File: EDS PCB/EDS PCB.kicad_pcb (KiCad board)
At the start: 2 copper layers, 100 x 100 mm, 1 part

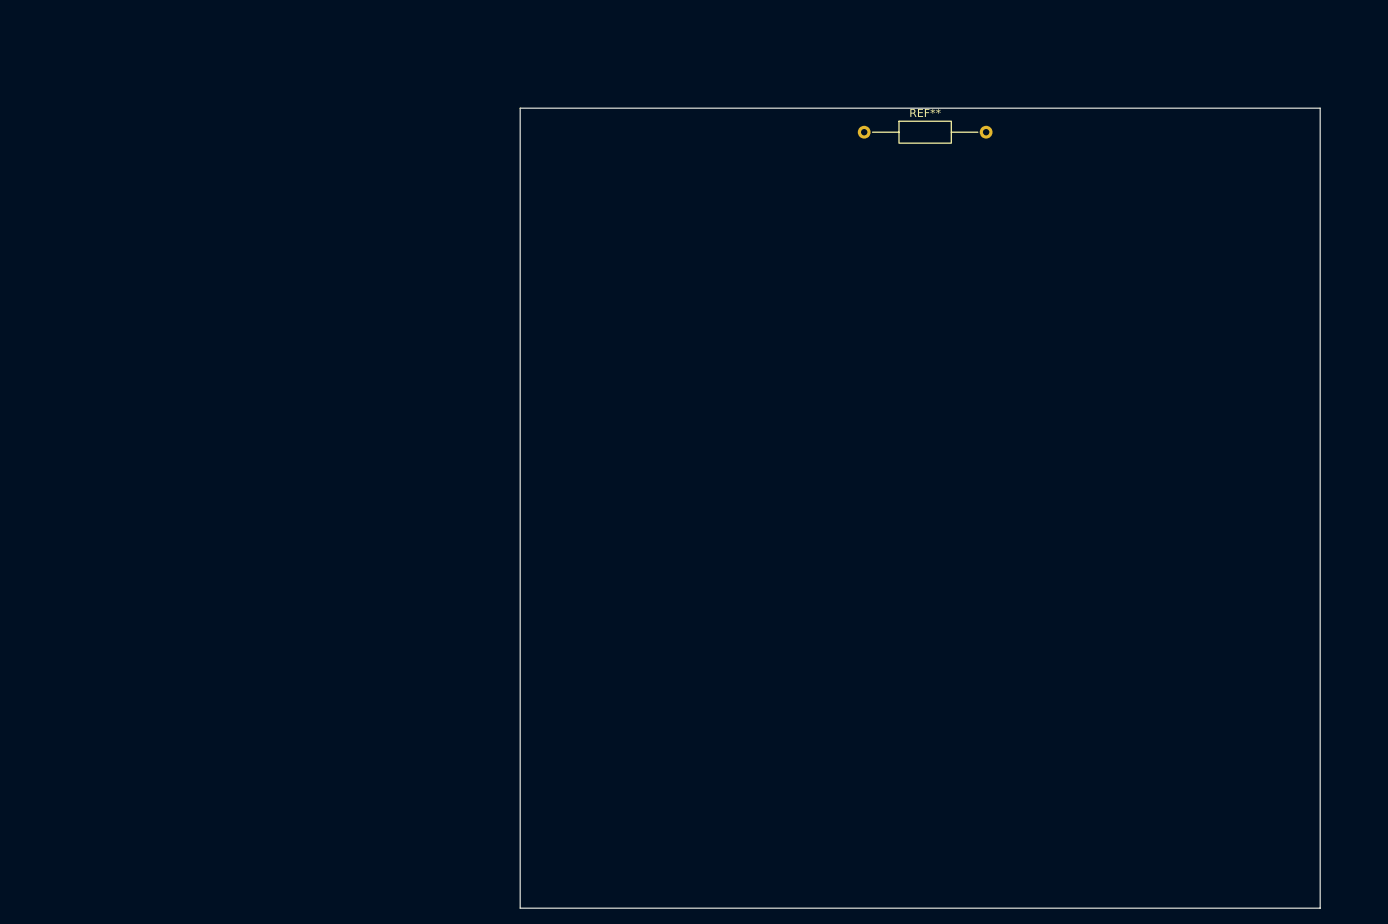
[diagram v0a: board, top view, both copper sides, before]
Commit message: EDS New shit
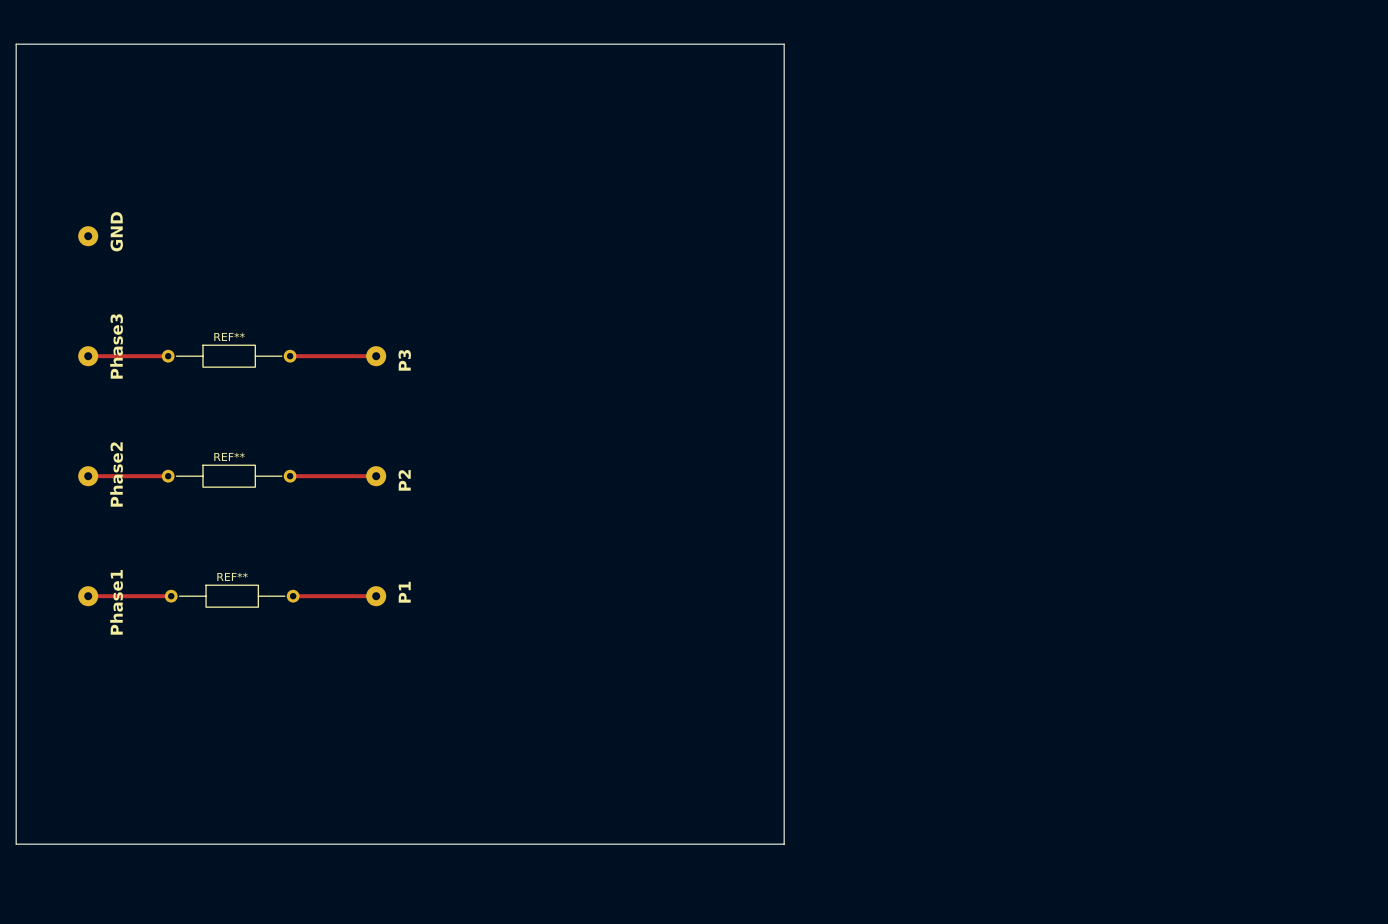
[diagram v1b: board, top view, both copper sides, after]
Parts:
- removed the REF** at (144.0, 41.0)
- added ?: , , F.Cu at (83.0, 84.0)
- added ?: , , F.Cu at (83.0, 69.0)
- added ?: , , F.Cu at (83.0, 99.0)
- added REF**: EDS_Input_Connector, EDS_Project_Library:EDS_Input_Connector, F.Cu at (47.0, 99.0)
- added REF**: R2, Resistor_THT:R_Axial_DIN0207_L6.3mm_D2.5mm_P15.24mm_Horizontal, F.Cu at (57.0, 84.0)
- added REF**: R3, Resistor_THT:R_Axial_DIN0207_L6.3mm_D2.5mm_P15.24mm_Horizontal, F.Cu at (57.0, 69.0)
- added REF**: R1, Resistor_THT:R_Axial_DIN0207_L6.3mm_D2.5mm_P15.24mm_Horizontal, F.Cu at (57.4, 99.0)
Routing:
- net (no net): track 0.00 -> 62.3 mm
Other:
- board size 100 x 100 mm -> 96 x 100 mm
- board text added: "P1"
- board text added: "P2"
- board text added: "P3"

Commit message: EDS Electrodes
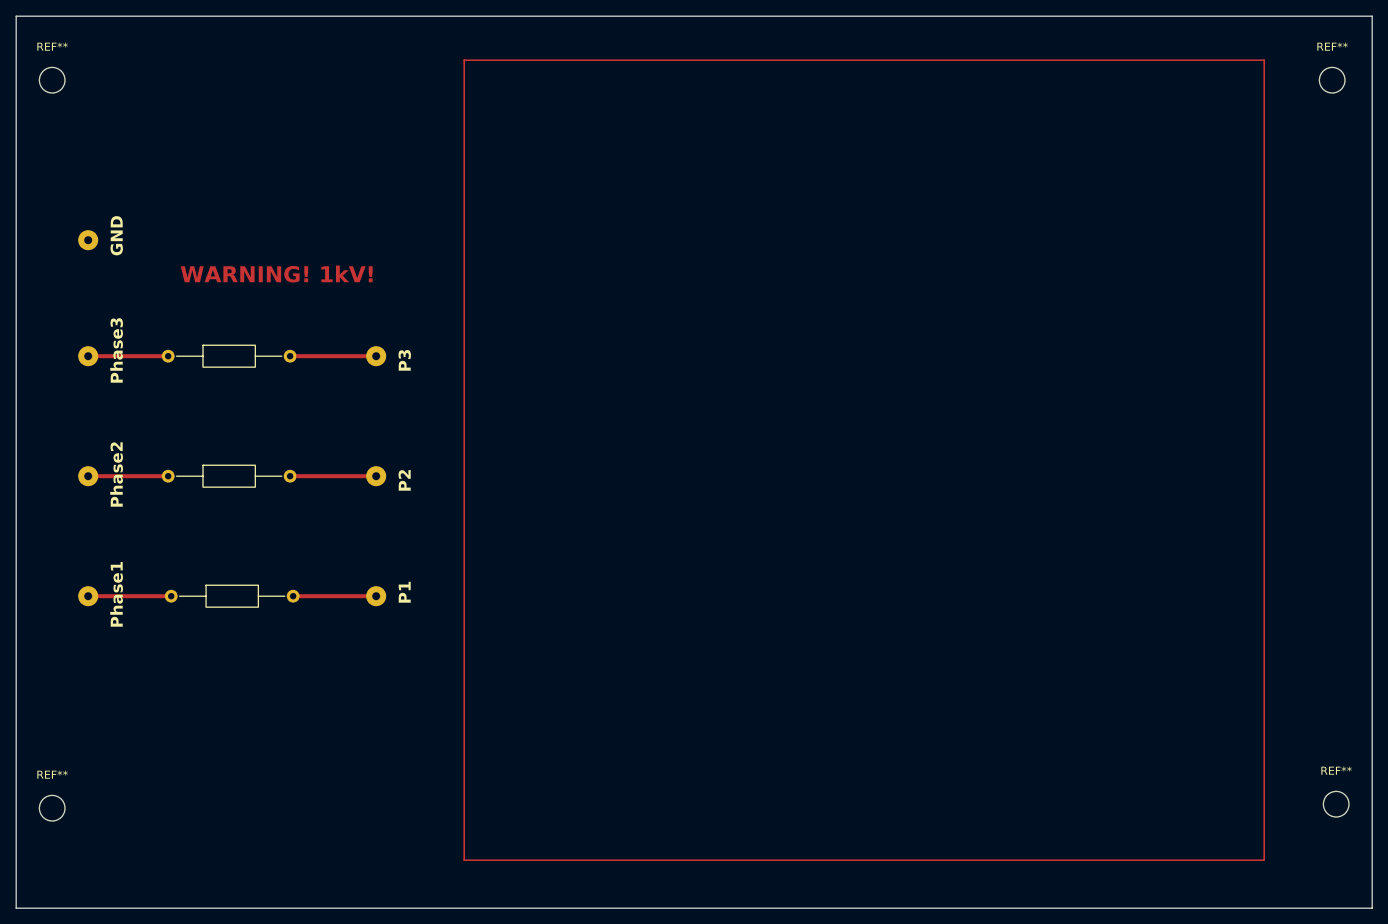
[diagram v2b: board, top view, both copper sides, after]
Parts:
- added ?: , clipboard:bf32c9e1-eea9-421a-b75f-750c3fb07239, F.Cu at (47.0, 54.5)
- added REF**: MountingHole_3.2mm_M3, MountingHole:MountingHole_3.2mm_M3, F.Cu at (203.0, 125.0)
- added REF**: MountingHole_3.2mm_M3, MountingHole:MountingHole_3.2mm_M3, F.Cu at (202.5, 34.5)
- added REF**: MountingHole_3.2mm_M3, MountingHole:MountingHole_3.2mm_M3, F.Cu at (42.5, 125.5)
- added REF**: MountingHole_3.2mm_M3, MountingHole:MountingHole_3.2mm_M3, F.Cu at (42.5, 34.5)
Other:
- board size 96 x 100 mm -> 169.5 x 111.5 mm
- board text added: "WARNING! 1kV!"
